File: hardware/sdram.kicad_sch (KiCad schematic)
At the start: 3 parts, among them U1 ECP5U_12_CABGA256, U7 W9825G6KH

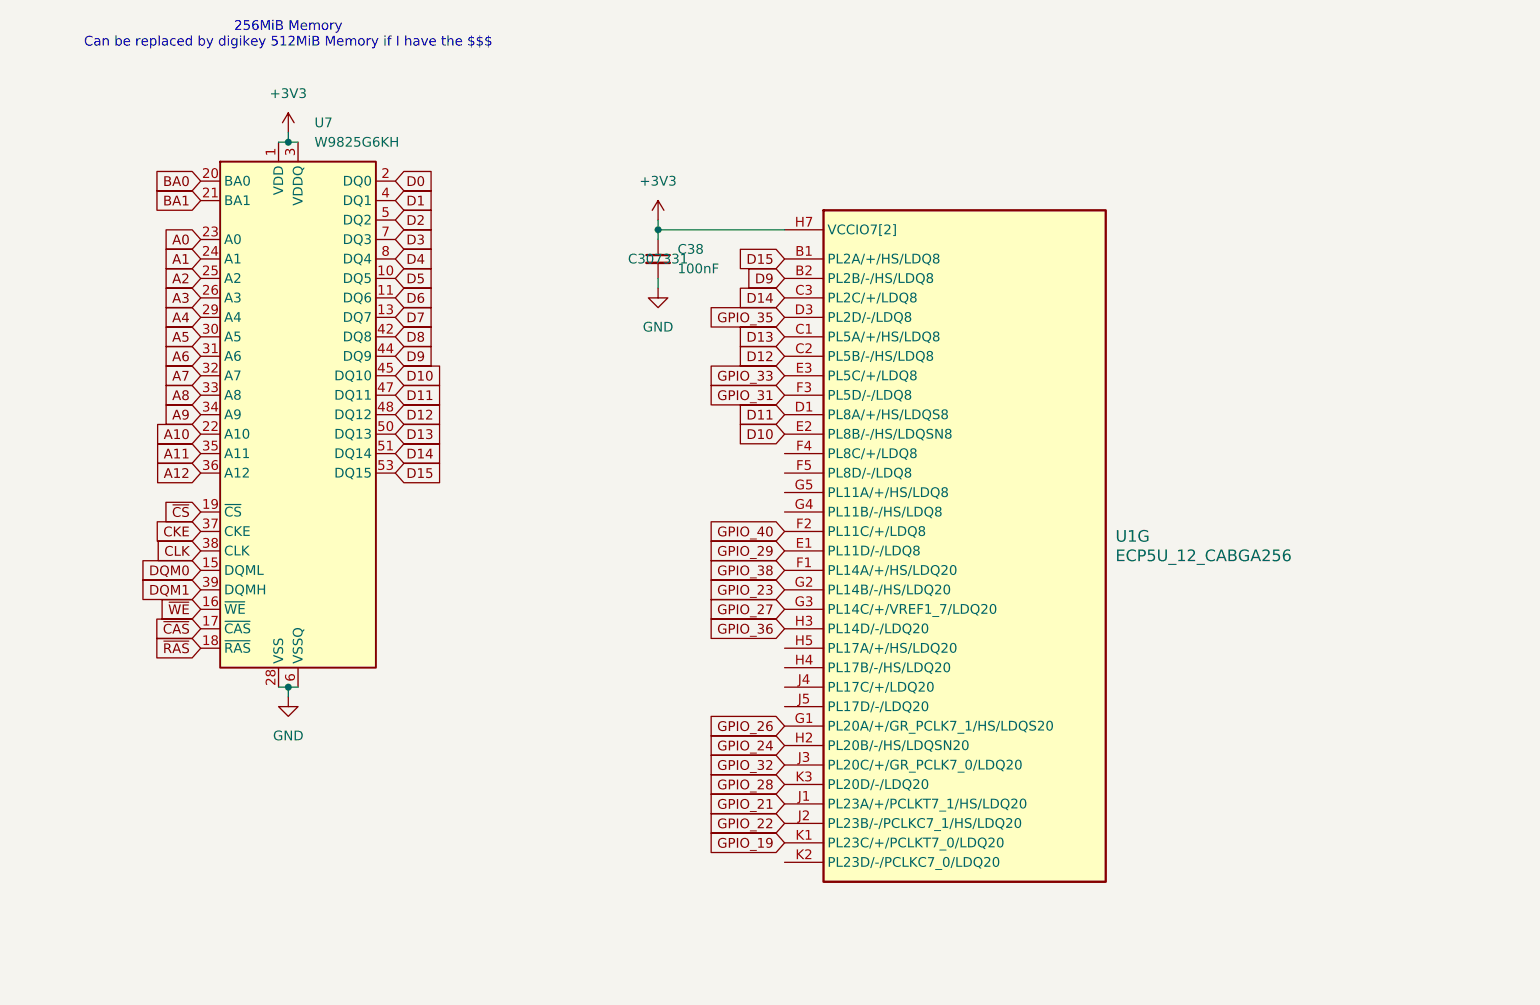
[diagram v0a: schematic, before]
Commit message: V1.0 Final Revision and Readme documentation
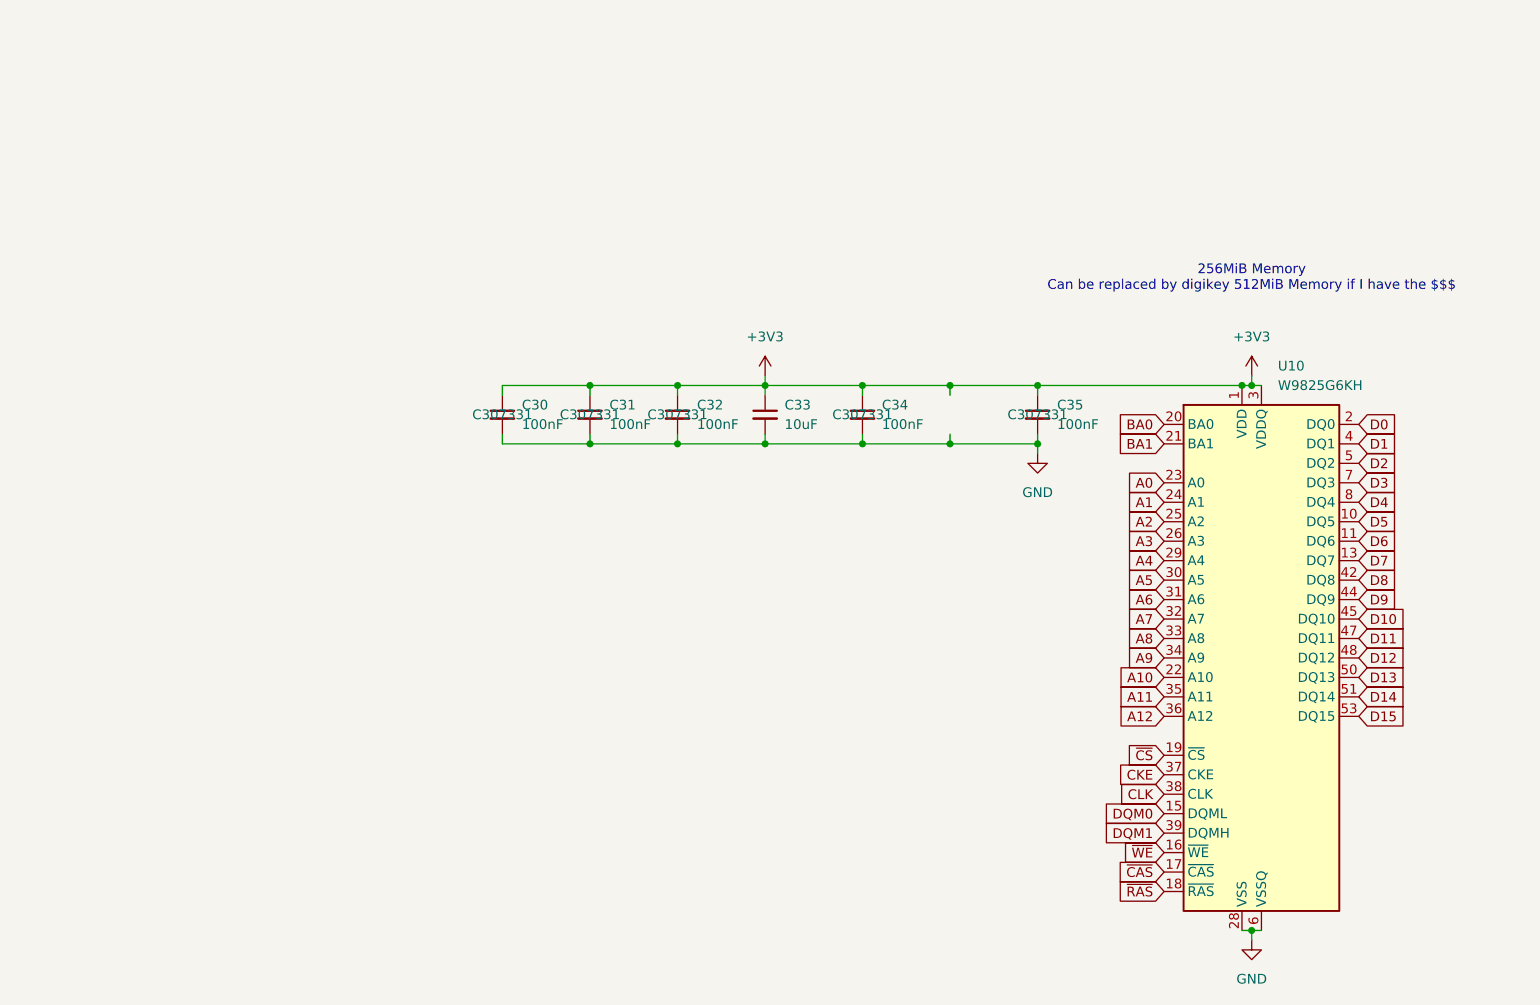
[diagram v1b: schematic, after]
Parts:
- removed C38: 100nF, Capacitor_SMD:C_0402_1005Metric, symbol Device:C_Small
- removed U1: ECP5U_12_CABGA256, Package_BGA:BGA-256_14.0x14.0mm_Layout16x16_P0.8mm_Ball0.45mm_Pad0.32mm_NSMD, symbol josh:ECP5U_12_CABGA256
- added C30, C31, C32, C34, C35: 100nF, Capacitor_SMD:C_0402_1005Metric, symbol Device:C_Small
- added C33: 10uF, Capacitor_SMD:C_0603_1608Metric, symbol Device:C_Small
- renumbered U7 to U10
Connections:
- net +3V3: now also C30.1, C31.1, C32.1, C33.1, C34.1, C35.1
- net GND: now also C30.2, C31.2, C32.2, C33.2, C34.2, C35.2
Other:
- moved on the sheet: U10
